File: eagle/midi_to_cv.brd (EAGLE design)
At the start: 100 x 80 mm, 66 parts, among them IC1 4093N, Q3 2N3904, Q4 2N3904, Q5 2N3904, Q6 2SK30, U1 ATMEGA328P_PDIP

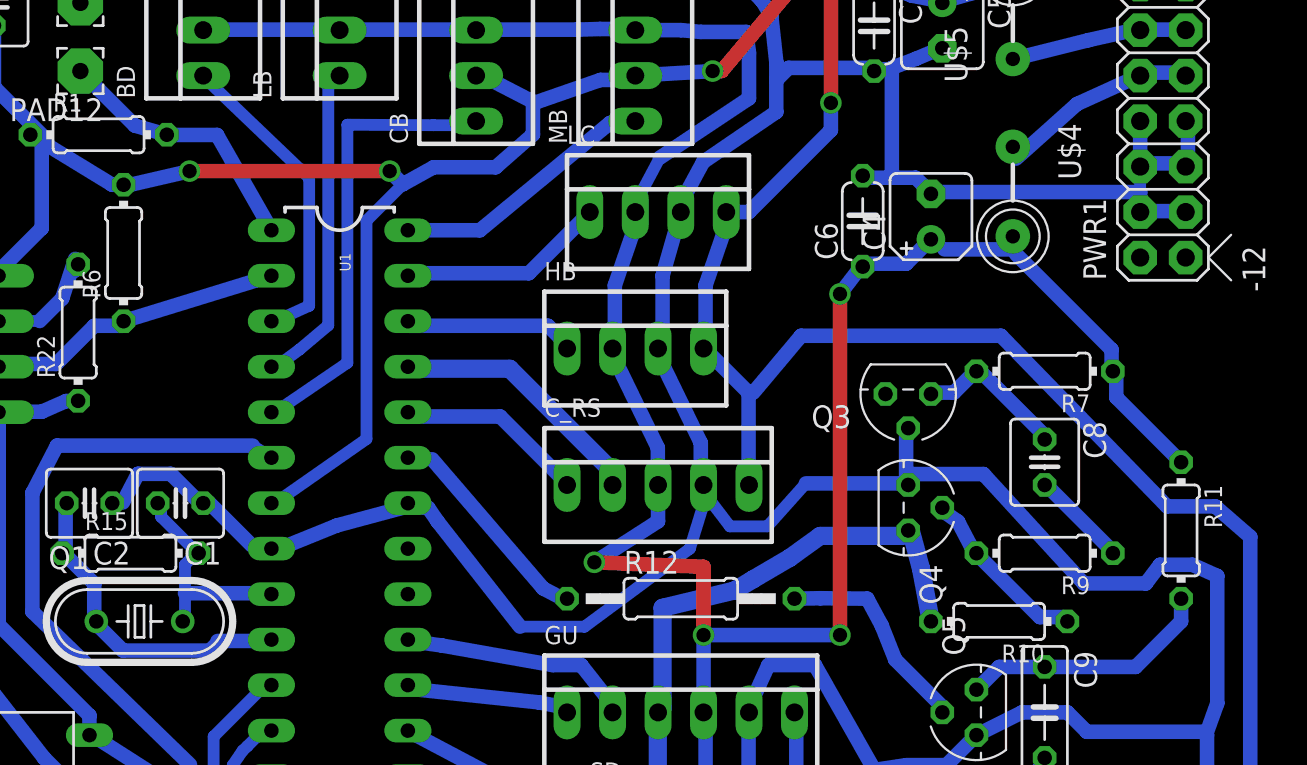
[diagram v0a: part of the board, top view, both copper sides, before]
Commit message: tweaks
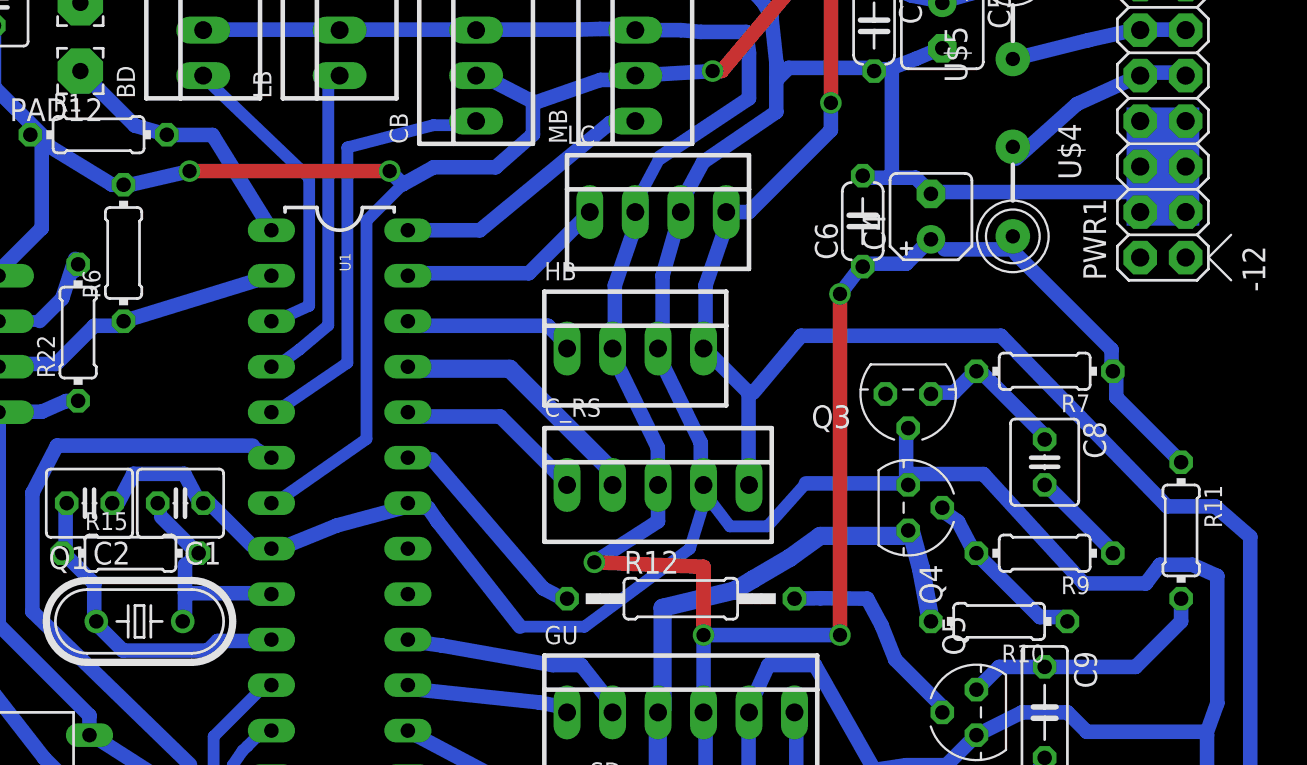
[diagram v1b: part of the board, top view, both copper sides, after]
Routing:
- net CB_TRIG: track 25.7 -> 24.5 mm
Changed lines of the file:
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@@
 <wire x1="100" y1="80" x2="0" y2="80" width="0" layer="20"/>
 <wire x1="0" y1="80" x2="0" y2="0" width="0" layer="20"/>
+<rectangle x1="84.582" y1="58.928" x2="88.646" y2="65.532" layer="16"/>
 </plain>
 <attributes>
@@
 <contactref element="C1" pad="2"/>
 <contactref element="R15" pad="2"/>
-<wire x1="32.004" y1="40.005" x2="32.004" y2="38.4048" width="0.6604" layer="16"/>
-<wire x1="32.004" y1="38.4048" x2="32.004" y2="37.0713" width="0.6604" layer="16"/>
+<wire x1="32.004" y1="40.005" x2="32.004" y2="38.4048" width="0.8128" layer="16"/>
+<wire x1="32.004" y1="38.4048" x2="32.004" y2="37.0713" width="0.8128" layer="16"/>
 <wire x1="32.5374" y1="40.5384" x2="32.004" y2="40.005" width="0.6604" layer="16"/>
 <wire x1="32.004" y1="37.0713" x2="31.877" y2="36.83" width="0.6604" layer="16"/>
 <wire x1="32.5374" y1="40.5384" x2="32.766" y2="40.64" width="0.6604" layer="16"/>
 <wire x1="30.6705" y1="42.672" x2="30.6705" y2="43.2054" width="0.6604" layer="16"/>
-<wire x1="32.5374" y1="40.8051" x2="30.6705" y2="42.672" width="0.6604" layer="16"/>
+<wire x1="32.5374" y1="40.8051" x2="30.6705" y2="42.672" width="0.8128" layer="16"/>
 <wire x1="30.6705" y1="43.2054" x2="30.48" y2="43.434" width="0.6604" layer="16"/>
 <wire x1="32.5374" y1="40.8051" x2="32.766" y2="40.64" width="0.6604" layer="16"/>
@@
 <wire x1="25.3365" y1="40.5384" x2="25.146" y2="40.64" width="0.6604" layer="16"/>
 <wire x1="33.8201" y1="35.7378" x2="36.8046" y2="35.7378" width="0.8128" layer="16"/>
-<wire x1="33.2867" y1="35.2044" x2="33.8201" y2="35.7378" width="0.6604" layer="16"/>
+<wire x1="33.2867" y1="35.2044" x2="33.8201" y2="35.7378" width="0.8128" layer="16"/>
 <wire x1="28.5369" y1="35.2044" x2="33.2867" y2="35.2044" width="0.8128" layer="16"/>
 <wire x1="27.2034" y1="36.5379" x2="28.5369" y2="35.2044" width="0.8128" layer="16"/>
@@
 <wire x1="31.115" y1="63.7413" x2="30.988" y2="64.008" width="0.6604" layer="16"/>
 <wire x1="36.8046" y1="58.674" x2="36.83" y2="58.674" width="0.6604" layer="16"/>
-<wire x1="31.4579" y1="63.9953" x2="33.7947" y2="63.9953" width="0.8128" layer="16"/>
-<wire x1="33.7947" y1="63.9953" x2="36.83" y2="58.674" width="0.8128" layer="16"/>
+<wire x1="31.4579" y1="63.9953" x2="33.5407" y2="63.9953" width="0.8128" layer="16"/>
+<wire x1="33.5407" y1="63.9953" x2="36.83" y2="58.674" width="0.8128" layer="16"/>
 <wire x1="30.988" y1="64.008" x2="29.21" y2="64.516" width="0.8128" layer="16"/>
 <wire x1="29.21" y1="64.516" x2="26.162" y2="67.564" width="0.8128" layer="16"/>
@@
 <wire x1="70.4088" y1="67.7418" x2="70.485" y2="67.564" width="0.6604" layer="16"/>
 <wire x1="48.5394" y1="72.2757" x2="48.26" y2="72.39" width="0.6604" layer="16"/>
-<wire x1="28.5369" y1="43.4721" x2="28.0035" y2="43.4721" width="0.6604" layer="16"/>
-<wire x1="29.3751" y1="45.0723" x2="28.5369" y2="43.4721" width="0.8128" layer="16"/>
-<wire x1="31.2039" y1="45.0723" x2="29.3751" y2="45.0723" width="0.8128" layer="16"/>
-<wire x1="32.8041" y1="43.4721" x2="31.2039" y2="45.0723" width="0.8128" layer="16"/>
+<wire x1="28.2829" y1="43.4721" x2="28.0035" y2="43.4721" width="0.6604" layer="16"/>
+<wire x1="29.1211" y1="45.0723" x2="28.2829" y2="43.4721" width="0.8128" layer="16"/>
+<wire x1="31.9659" y1="45.0723" x2="29.1211" y2="45.0723" width="0.8128" layer="16"/>
+<wire x1="32.8041" y1="43.4721" x2="31.9659" y2="45.0723" width="0.8128" layer="16"/>
 <wire x1="28.0035" y1="43.4721" x2="27.94" y2="43.434" width="0.6604" layer="16"/>
 <wire x1="32.8041" y1="43.4721" x2="33.02" y2="43.434" width="0.6604" layer="16"/>
@@
 <contactref element="U1" pad="5"/>
 <wire x1="41.0718" y1="51.2699" x2="37.0713" y2="48.5394" width="0.6604" layer="16"/>
-<wire x1="41.0718" y1="64.5668" x2="41.0718" y2="51.2699" width="0.6604" layer="16"/>
-<wire x1="45.8724" y1="64.5414" x2="41.0718" y2="64.5668" width="0.6604" layer="16"/>
+<wire x1="41.0718" y1="63.2968" x2="41.0718" y2="51.2699" width="0.6604" layer="16"/>
+<wire x1="45.8724" y1="64.5414" x2="41.0718" y2="63.2968" width="0.6604" layer="16"/>
 <wire x1="48.006" y1="64.5414" x2="45.8724" y2="64.5414" width="0.6604" layer="16"/>
 <wire x1="37.0713" y1="48.5394" x2="36.83" y2="48.514" width="0.6604" layer="16"/>
